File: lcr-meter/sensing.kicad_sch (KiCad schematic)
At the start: 37 parts, among them J4 Conn_01x04, U10 AMP03GPZ, U11 TMUX1101DCK, U12 TMUX1101DCK, U14 LF353N/NOPB, U16 LF353N/NOPB, U2 AMP03GPZ, U21 AMP03GPZ, U3 AMP03GPZ, U8 TMUX1101DCK, U9 TMUX1101DCK

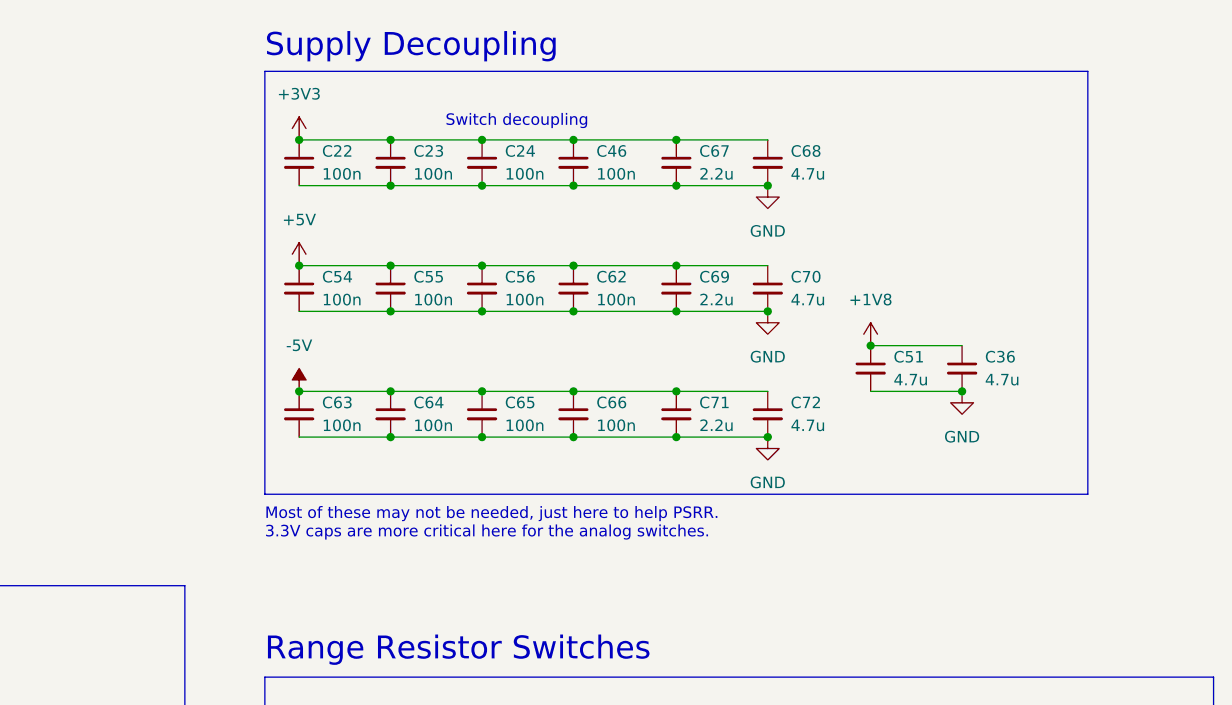
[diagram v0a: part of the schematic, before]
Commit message: PCB updates
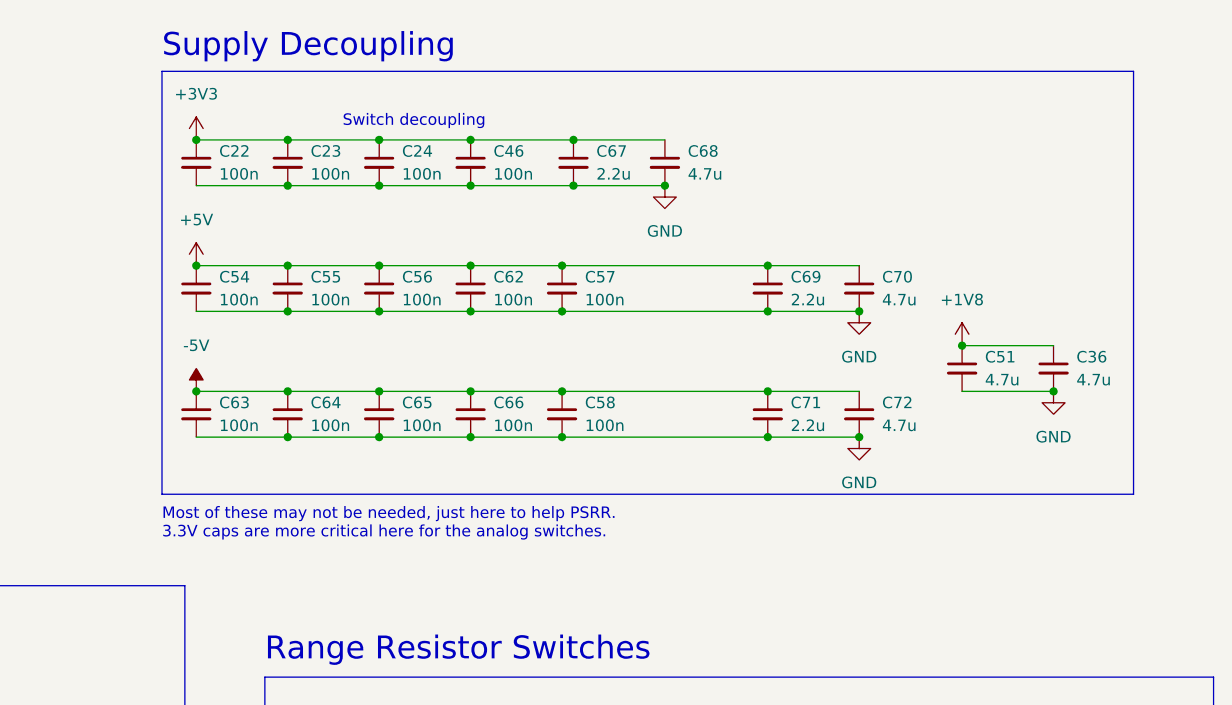
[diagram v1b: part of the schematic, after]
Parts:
- added C57, C58: 100n, Capacitor_SMD:C_0402_1005Metric, symbol Device:C_Small
- U11, U12, U8, U9: footprint Package_TO_SOT_SMD:SOT-23-5 -> Package_TO_SOT_SMD:SOT-353_SC-70-5
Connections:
- net +5V: now also C57.1
- net -5V: now also C58.1
- net GND: now also C57.2, C58.2
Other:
- moved on the sheet: C22, C23, C24, C36, C46, C51, C54, C55, C56, C62, C63, C64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
